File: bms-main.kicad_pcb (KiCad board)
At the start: 2 copper layers, 67 parts, among them J1 CONN HEADER VERT 2POS 1.5MM, J2 CONN HEADER VERT 2POS 1.5MM, J3 CONN HEADER VERT 2POS 1.5MM, J4 CONN HEADER VERT 4POS 2.5MM, J5 PIN HEADER 2.54MM PITCH STR D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, J6 XT60PW-M, J7 XT60PW-M, U1 TLE9015DQUXUMA1, U2 STM32L433CCU6, U3 IC TRANSCEIVER 1/1 8SO, U4 INA181A3IDBVR, X1 CRYSTAL 32.0000MHZ 10PF SMD

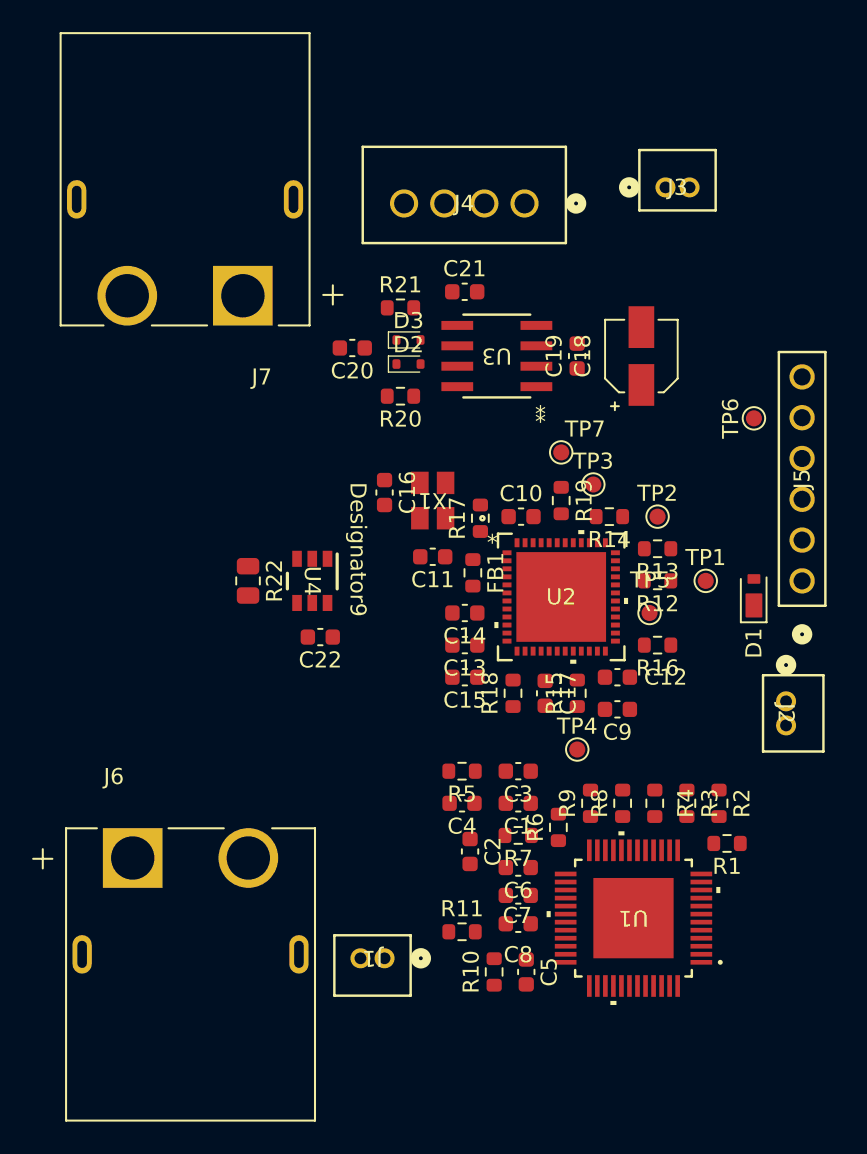
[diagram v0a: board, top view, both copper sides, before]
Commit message: 2 layer
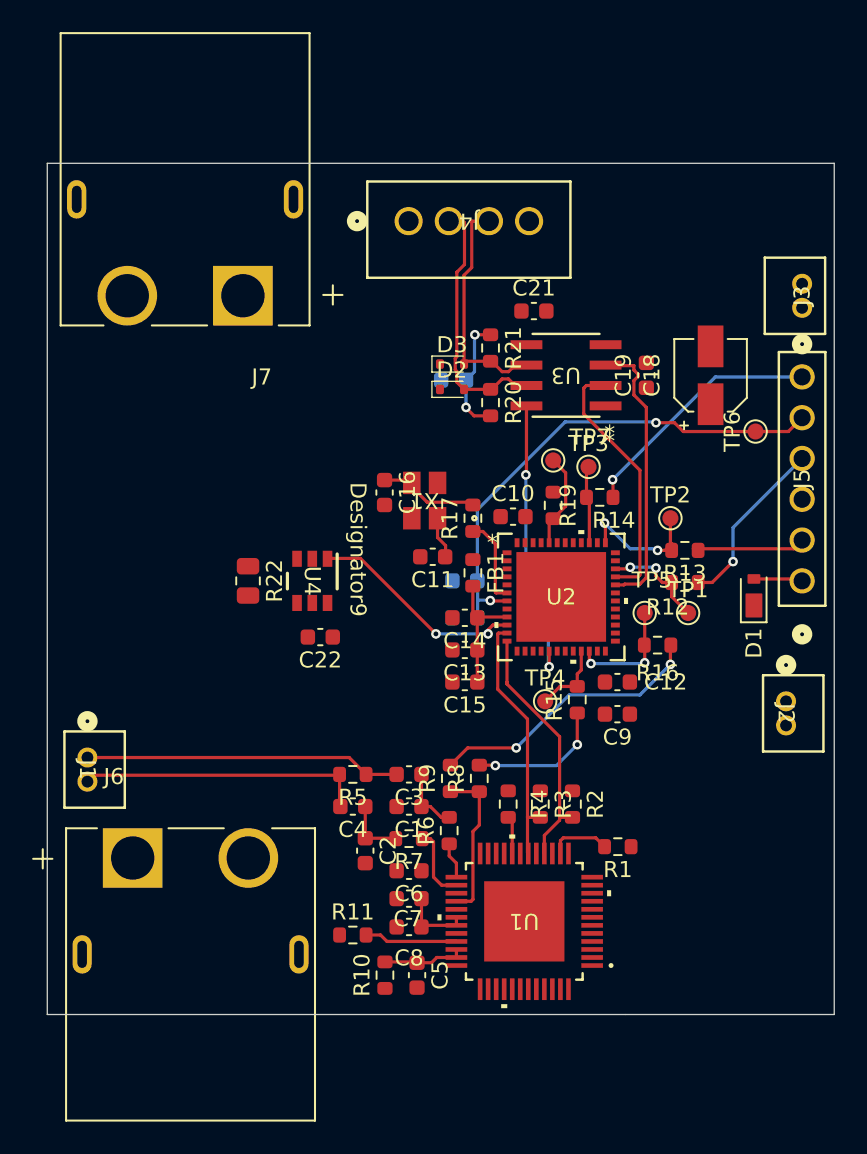
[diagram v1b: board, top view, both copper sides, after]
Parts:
- C17, C20, R18: moved to B.Cu
- moved J1 22.3 mm to (143.5, 71.5), turned to -90 degrees
- moved J3 11.3 mm to (188.0, 43.5), turned to 90 degrees
- moved R2 9.13 mm to (173.7, 74.4)
- moved R3 9.13 mm to (171.7, 74.4)
- moved R4 9.13 mm to (169.7, 74.4)
- moved R8 9.06 mm to (167.9, 72.8)
- moved R9 8.86 mm to (166.1, 72.8)
- moved C17 8.60 mm to (167.0, 60.5), turned to 180 degrees
- moved J4 7.30 mm to (163.5, 38.1), turned to 180 degrees
- moved U1 6.80 mm to (170.7, 81.7)
- moved C1 6.80 mm to (163.5, 74.5)
- moved C3 6.80 mm to (163.5, 72.5)
- moved C4 6.80 mm to (160.0, 74.5)
- moved C5 6.80 mm to (164.0, 85.0)
- moved C6 6.80 mm to (163.5, 78.5)
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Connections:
- net /CANTranceiver/CANH_P renamed /CANTranceiver/CAN_P
- net /CANTranceiver/CANL_N renamed /CANTranceiver/CAN_N
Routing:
- net /STM/NRST: track 0.00 -> 31.5 mm, vias 0 -> 2
- net /isoUARTTranceiver/IFH_H: track 0.00 -> 19.7 mm
- net /isoUARTTranceiver/IFH_L: track 0.00 -> 17.9 mm
- net /CANTranceiver/STBY: track 0.00 -> 17.8 mm, vias 0 -> 2
- net /CANTranceiver/RXD: track 0.00 -> 17.6 mm
- net /STM/PB11/UART4_RX: track 0.00 -> 17.5 mm, vias 0 -> 2
- net /CANTranceiver/CAN_P: track 0.00 -> 16.2 mm
- net /CANTranceiver/TXD: track 0.00 -> 16.1 mm
- net /isoUARTTranceiver/ERRQ_RES: track 0.00 -> 16.0 mm
- net /isoUARTTranceiver/ERRQ_EXT: track 0.00 -> 15.9 mm
- net /STM/SWO: track 0.00 -> 15.6 mm, vias 0 -> 1
- net /CANTranceiver/CAN_N: track 0.00 -> 14.7 mm
- net /CurrentSense/C_Sense: track 0.00 -> 13.5 mm, vias 0 -> 2
- net /STM/SWDIO: track 0.00 -> 10.9 mm, vias 0 -> 1
- net /isoUARTTranceiver/UART_LS: track 0.00 -> 9.75 mm
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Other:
- board outline added: 49 x 53 mm
